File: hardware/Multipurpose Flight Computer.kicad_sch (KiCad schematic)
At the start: 79 parts, among them J1 Screw_Terminal_01x02, J2 Conn_01x03, J3 Conn_01x03, SW1 TS-1088-AR02016, SW2 TS-1088-AR02016, U1 BQ25883RGER, U2 ICM-45686, U3 STM32F722RETx, U4 BMP580, U5 TPS63070RNMR, U6 LMR51430, X1 X322525MOB4SI, X2 Q13FC1350000400

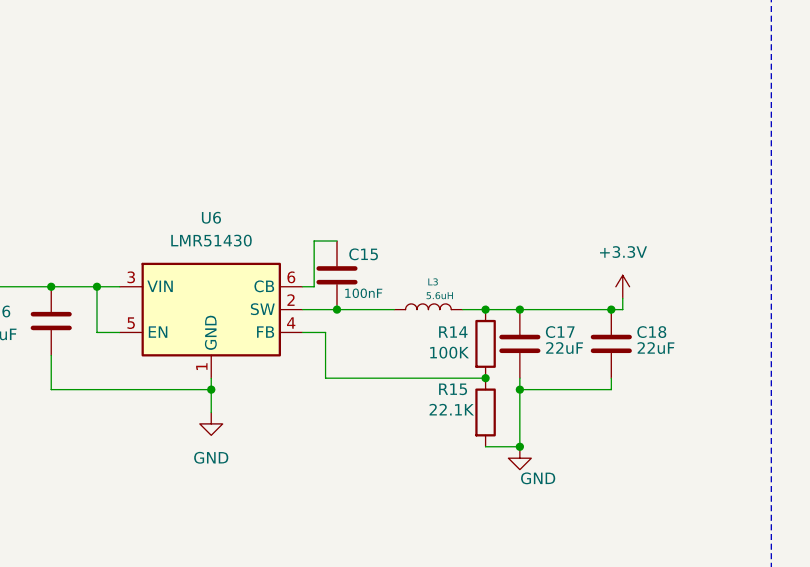
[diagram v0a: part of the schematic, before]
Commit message: Updating KiCad
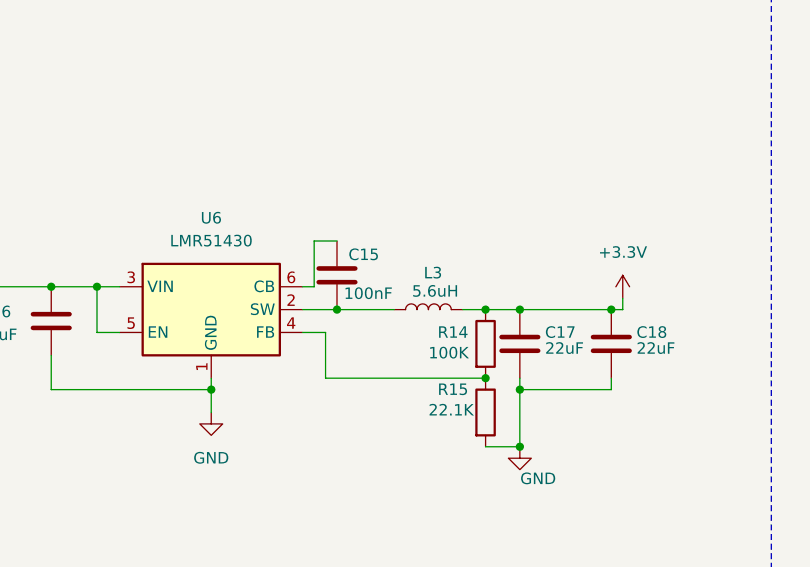
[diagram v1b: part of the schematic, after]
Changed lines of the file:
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@@
 			(effects
 				(font
-					(size 1.016 1.016)
+					(size 1.27 1.27)
 				)
 				(justify left)
@@
 		(dnp no)
 		(property "Reference" "L3"
-			(at 81.788 236.982 90)
-			(effects
-				(font
-					(size 0.762 0.762)
+			(at 81.788 235.966 90)
+			(effects
+				(font
+					(size 1.27 1.27)
 				)
 			)
 		)
 		(property "Value" "5.6uH"
-			(at 82.55 238.506 90)
-			(effects
-				(font
-					(size 0.762 0.762)
-				)
-			)
+			(at 82.042 237.998 90)
+			(effects
+				(font
+					(size 1.27 1.27)
+				)
+			)
